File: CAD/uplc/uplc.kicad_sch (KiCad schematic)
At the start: 34 parts, among them J1 Conn_01x06_Pin, J2 SM12B-GHS-TB(LF)(SN), K1 G6K-2F-Y, K2 G6K-2F-Y, U1 DS8242-33S5, U3 ESP32-C3-WROOM-02, U5 TBD62003AFWG, Y1 32.568khz

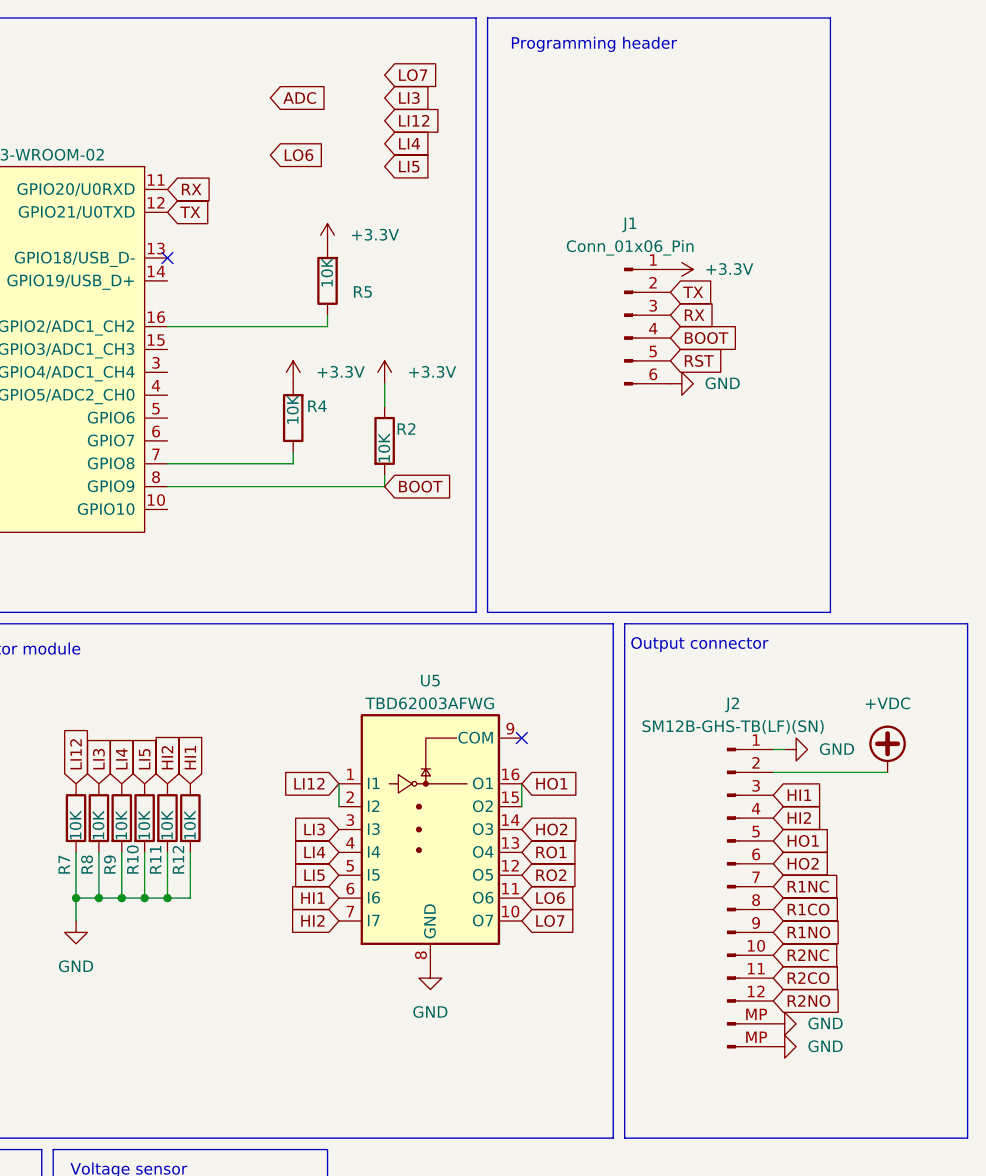
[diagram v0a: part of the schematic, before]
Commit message: wip
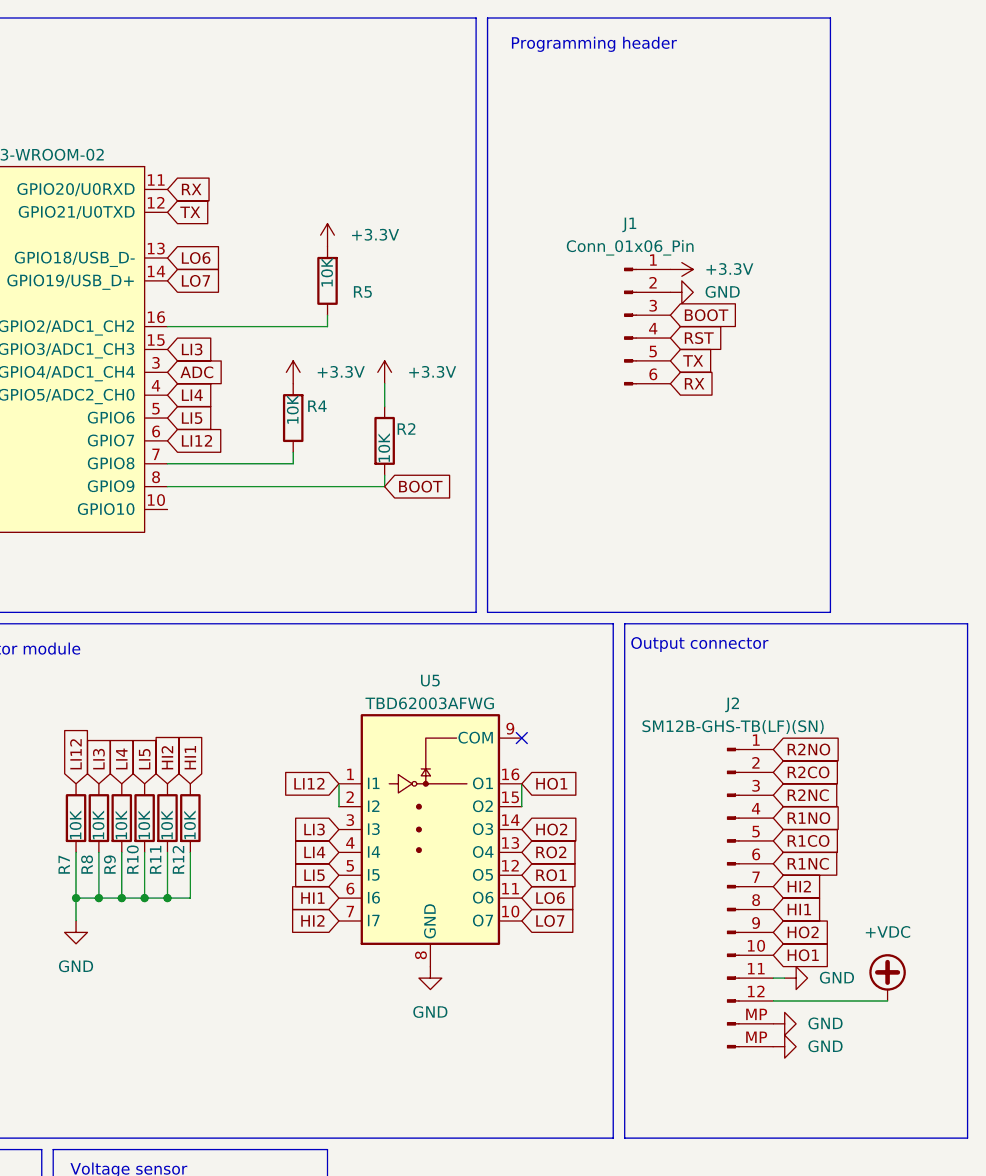
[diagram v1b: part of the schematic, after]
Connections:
- net +VDC: now also J2.12 (Pin_12); no longer J2.2 (Pin_2)
- net ADC: now also U3.3 (GPIO4/ADC1_CH4)
- net BOOT: now also J1.3 (Pin_3); no longer J1.4 (Pin_4)
- net GND: now also J1.2 (Pin_2), J2.11 (Pin_11); no longer J1.6 (Pin_6), J2.1 (Pin_1)
- net HI1: now also J2.8 (Pin_8); no longer J2.3 (Pin_3)
- net HI2: now also J2.7 (Pin_7); no longer J2.4 (Pin_4)
- net HO1: now also J2.10 (Pin_10); no longer J2.5 (Pin_5)
- net HO2: now also J2.9 (Pin_9); no longer J2.6 (Pin_6)
- net LI12: now also U3.6 (GPIO7)
- net LI3: now also U3.15 (GPIO3/ADC1_CH3)
- net LI4: now also U3.4 (GPIO5/ADC2_CH0)
- net LI5: now also U3.5 (GPIO6)
- net LO6: now also U3.13 (GPIO18/USB_D-)
- net LO7: now also U3.14 (GPIO19/USB_D+)
- net R1CO: now also J2.5 (Pin_5); no longer J2.8 (Pin_8)
- net R1NC: now also J2.6 (Pin_6); no longer J2.7 (Pin_7)
- net R1NO: now also J2.4 (Pin_4); no longer J2.9 (Pin_9)
- net R2CO: now also J2.2 (Pin_2); no longer J2.11 (Pin_11)
- net R2NC: now also J2.3 (Pin_3); no longer J2.10 (Pin_10)
- net R2NO: now also J2.1 (Pin_1); no longer J2.12 (Pin_12)
- net RO1: now also U5.12 (O5); no longer U5.13 (O4)
- net RO2: now also U5.13 (O4); no longer U5.12 (O5)
- net RST: now also J1.4 (Pin_4); no longer J1.5 (Pin_5)
- net RX: now also J1.6 (Pin_6); no longer J1.3 (Pin_3)
- net TX: now also J1.5 (Pin_5); no longer J1.2 (Pin_2)
- no-connect marks 3 -> 2
